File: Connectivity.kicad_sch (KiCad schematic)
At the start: 5 parts, among them U1 ESP32-C3-DevKitM-1

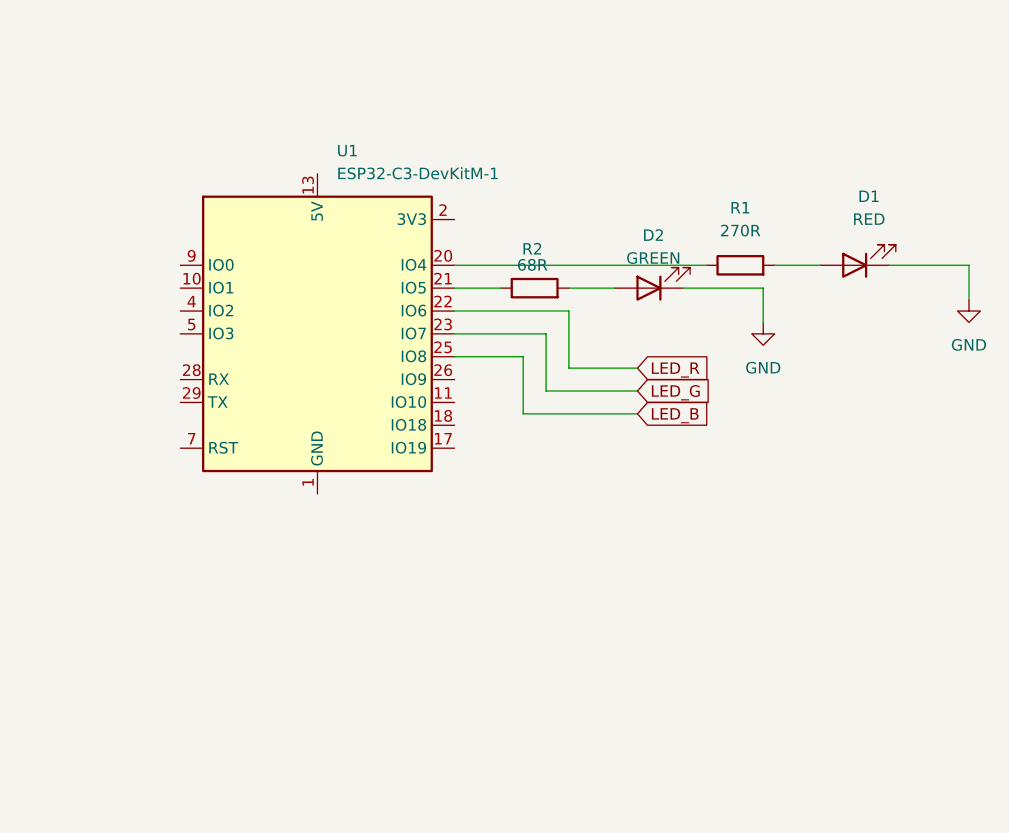
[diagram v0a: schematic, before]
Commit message: Lesson 4 - Power Supply
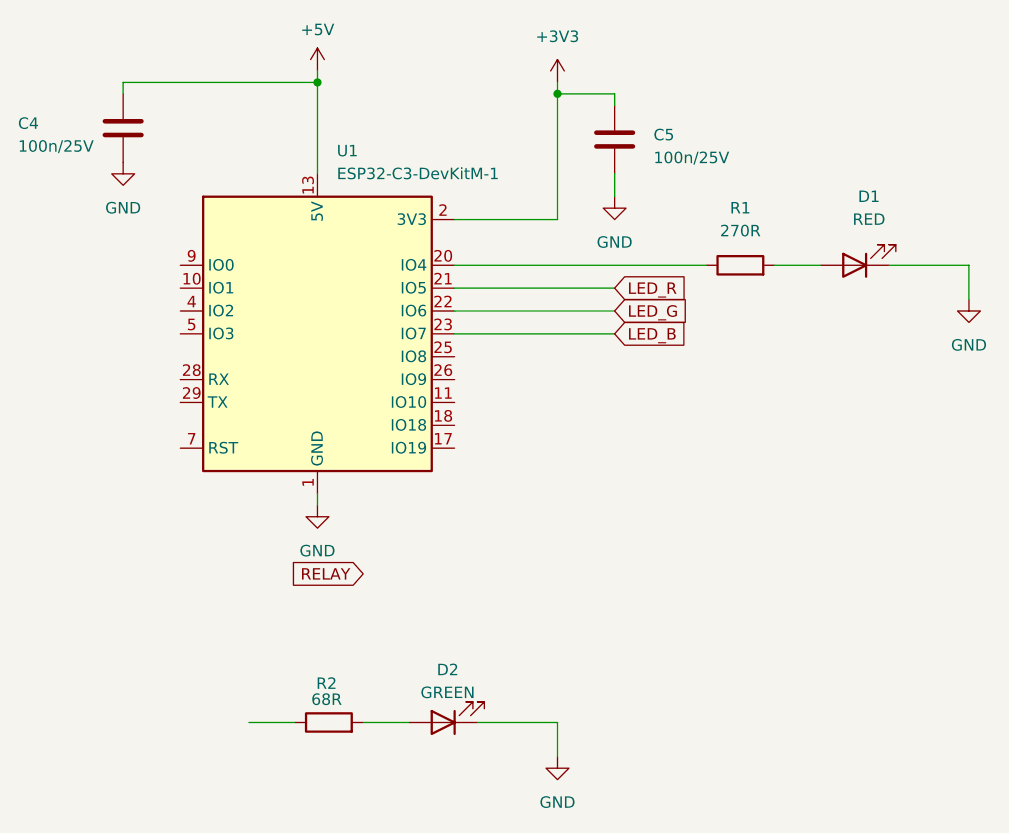
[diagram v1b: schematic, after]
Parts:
- added C4, C5: 100n/25V, Capacitor_SMD:C_1206_3216Metric, symbol Device:C
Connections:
- net GND: now also U1.1 (GND), U1.12 (GND), U1.15 (GND), U1.16 (GND), U1.19 (GND), U1.24 (GND), U1.27 (GND), U1.30 (GND), U1.6 (GND), U1.8 (GND), C4.2, C5.2
- net LED_B: now also U1.23 (IO7); no longer U1.25 (IO8)
- net LED_G: now also U1.22 (IO6); no longer U1.23 (IO7)
- net LED_R: now also U1.21 (IO5); no longer U1.22 (IO6)
- net at R2.1: no longer U1.21 (IO5)
- net +5V: now reaches U1.13 (5V), U1.14 (5V)
- net +5V: now also C4.1
- net +3V3: now reaches U1.2 (3V3), U1.3 (3V3)
- net +3V3: now also C5.1
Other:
- moved on the sheet: D2, R2
